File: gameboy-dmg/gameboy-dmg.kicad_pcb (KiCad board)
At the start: 2 copper layers, 82 x 63.5 mm, 29 parts, among them J1 Conn_01x02, J2 Conn_01x06, J3 Conn_01x02, U1 MCP23017_SO

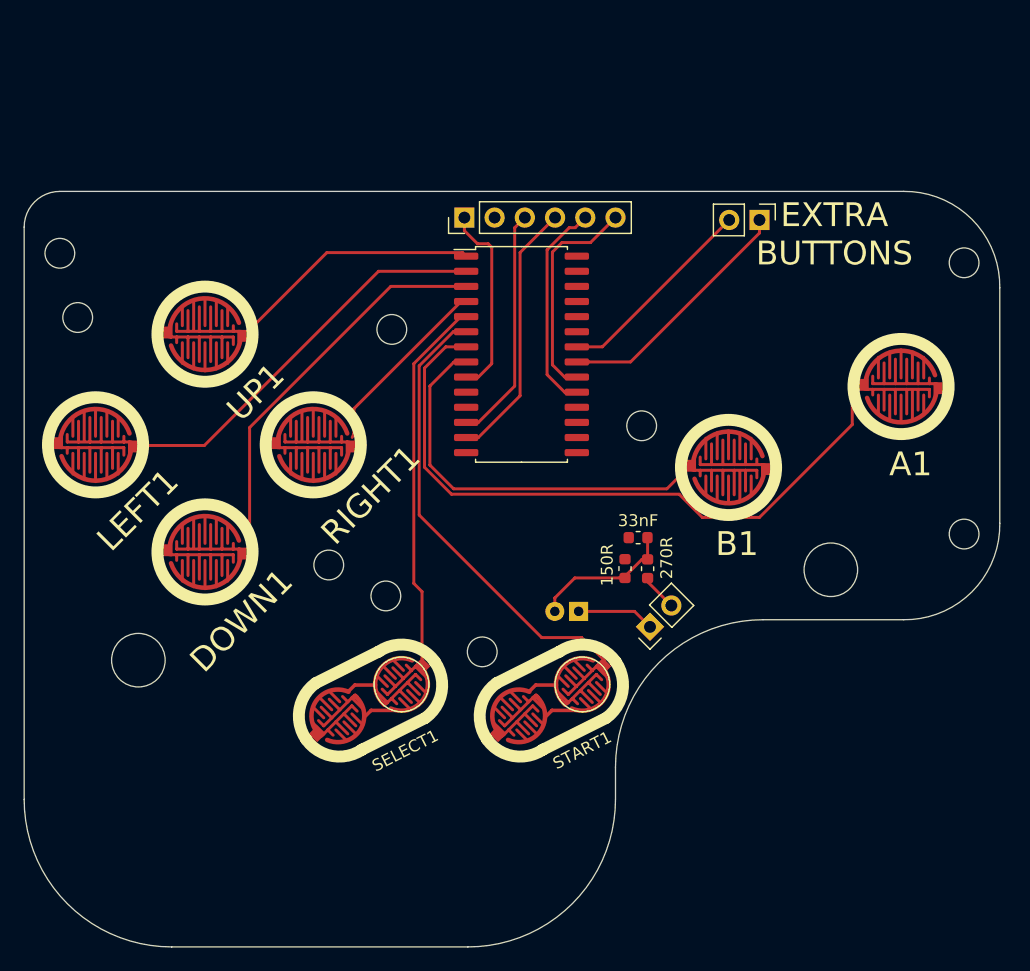
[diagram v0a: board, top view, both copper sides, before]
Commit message: Added some more bits
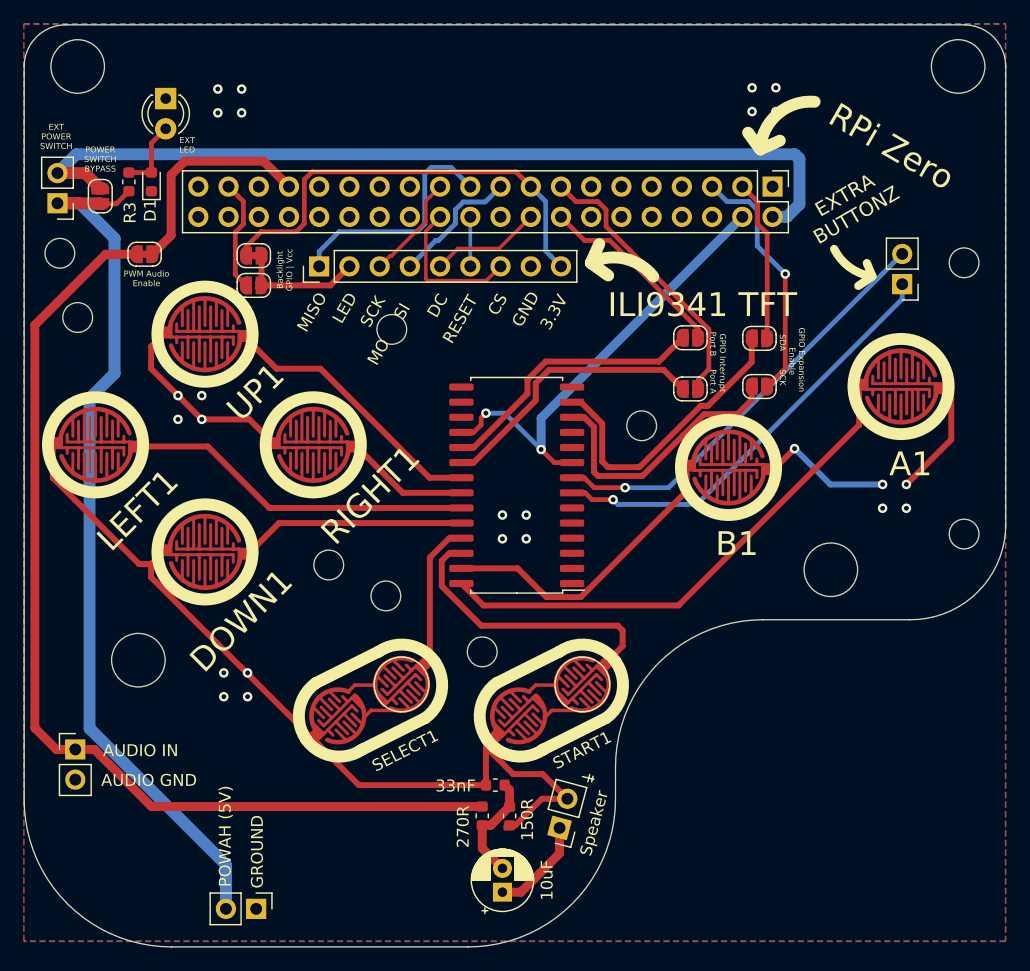
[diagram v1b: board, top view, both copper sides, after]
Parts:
- added D1: LED, LED_SMD:LED_0603_1608Metric, F.Cu at (133.7, 72.2)
- added D2: LED, LED_THT:LED_D3.0mm, F.Cu at (134.9, 65.2)
- added J4: Conn_01x02, Connector_PinHeader_2.54mm:PinHeader_1x02_P2.54mm_Vertical, F.Cu at (127.3, 119.9)
- added J5: Raspberry_Pi_2_3, Connector_PinHeader_2.54mm:PinHeader_2x20_P2.54mm_Vertical, F.Cu at (185.9, 72.6)
- added J6: Conn_01x09, Connector_PinHeader_2.54mm:PinHeader_1x09_P2.54mm_Vertical, F.Cu at (147.8, 79.3)
- added JP1: SolderJumper_2_Bridged, Jumper:SolderJumper-2_P1.3mm_Bridged_RoundedPad1.0x1.5mm, F.Cu at (133.1, 78.3)
- added JP2: SolderJumper_2_Open, Jumper:SolderJumper-2_P1.3mm_Open_RoundedPad1.0x1.5mm, F.Cu at (184.8, 89.4)
- added JP3: SolderJumper_2_Open, Jumper:SolderJumper-2_P1.3mm_Open_RoundedPad1.0x1.5mm, F.Cu at (184.8, 85.3)
- added JP4: SolderJumper_2_Open, Jumper:SolderJumper-2_P1.3mm_Open_RoundedPad1.0x1.5mm, F.Cu at (179.0, 85.3)
- added JP5: SolderJumper_2_Open, Jumper:SolderJumper-2_P1.3mm_Open_RoundedPad1.0x1.5mm, F.Cu at (179.0, 89.6)
- added JP6: SolderJumper_2_Open, Jumper:SolderJumper-2_P1.3mm_Open_RoundedPad1.0x1.5mm, F.Cu at (142.3, 80.9)
- added JP7: SolderJumper_2_Bridged, Jumper:SolderJumper-2_P1.3mm_Bridged_RoundedPad1.0x1.5mm, F.Cu at (142.3, 78.4)
- added JP8: SolderJumper_2_Open, Jumper:SolderJumper-2_P1.3mm_Open_RoundedPad1.0x1.5mm, F.Cu at (129.4, 73.4)
- added R3: R_Small, Resistor_SMD:R_0603_1608Metric, F.Cu at (131.8, 72.2)
- added REF**: MountingHole_4.5mm, MountingHole:MountingHole_4.5mm, F.Cu at (127.5, 62.5)
- added REF**: MountingHole_4.5mm, MountingHole:MountingHole_4.5mm, F.Cu at (201.5, 62.5)
- added SW1: SW_DIP_x01, Connector_PinHeader_2.54mm:PinHeader_1x02_P2.54mm_Vertical, F.Cu at (125.8, 74.0)
- C2: moved to F.Cu
- J2: value Conn_01x06 -> Conn_01x02; footprint Connector_PinHeader_2.54mm:PinHeader_1x06_P2.54mm_Vertical -> Connector_PinHeader_2.54mm:PinHeader_1x02_P2.54mm_Vertical
- moved J2 60.7 mm to (142.5, 133.3), turned to 270 degrees
- moved R1 25.0 mm to (161.5, 125.5), turned to 90 degrees
- moved C2 24.5 mm to (163.2, 131.9), turned to 90 degrees
- moved C1 24.0 mm to (162.6, 122.9)
- moved R2 23.0 mm to (163.8, 125.5), turned to 90 degrees
- moved J1 18.5 mm to (168.0, 126.5), turned to 165 degrees
- moved J3 13.2 mm to (196.8, 80.8), turned to 180 degrees
- moved U1 11.0 mm to (164.4, 97.7), turned to 180 degrees
- moved G*** 6.02 mm to (176.5, 107.0)
- moved G*** 0.22 mm to (135.9, 106.7)
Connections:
- J1 pad 2: /PWM_IN -> GND
- J2 pad 1: +5V -> GND
- J2 pad 2: GND -> Net-(J2-Pad2)
- U1 pad 1: /UP -> Net-(U1-Pad1)
- U1 pad 12: Net-(J2-Pad3) -> /GPIO_SCK
- U1 pad 13: Net-(J2-Pad4) -> /GPIO_SDA
- U1 pad 19: Net-(J2-Pad5) -> /GPIO_INTB
- U1 pad 2: /LEFT -> Net-(U1-Pad2)
- U1 pad 20: Net-(J2-Pad6) -> /GPIO_INTA
- U1 pad 21: Net-(J3-Pad1) -> /UP
- U1 pad 22: Net-(J3-Pad2) -> /RIGHT
- U1 pad 23: Net-(U1-Pad23) -> /LEFT
- U1 pad 24: Net-(U1-Pad24) -> /DOWN
- U1 pad 25: Net-(U1-Pad25) -> /SELECT
- U1 pad 26: Net-(U1-Pad26) -> /START
- U1 pad 27: Net-(U1-Pad27) -> /B
- U1 pad 28: Net-(U1-Pad28) -> /A
- U1 pad 3: /DOWN -> Net-(U1-Pad3)
- U1 pad 4: /RIGHT -> Net-(U1-Pad4)
- U1 pad 5: /SELECT -> Net-(U1-Pad5)
- U1 pad 6: /START -> Net-(U1-Pad6)
- U1 pad 7: /A -> Net-(J3-Pad1)
- U1 pad 8: /B -> Net-(J3-Pad2)
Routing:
- net GND: track 0.00 -> 108.1 mm, vias 0 -> 25
- net +5V: track 16.4 -> 112.4 mm, vias 0 -> 2
- net /PWM_IN: track 3.13 -> 85.2 mm
- net Net-(J2-Pad2): track 0.00 -> 74.4 mm
- net +3V3: track 0.00 -> 37.7 mm
- net /GPIO_SDA: track 0.00 -> 24.9 mm
- net /GPIO_INTA_PI: track 0.00 -> 23.6 mm
- net /GPIO_INTA: track 0.00 -> 23.3 mm
- net /GPIO_SCK: track 0.00 -> 23.1 mm
- net /GPIO_INTB: track 0.00 -> 23.1 mm
- net Net-(J2-Pad4): track 22.2 -> 0.00 mm
- net /GPIO_SCK_PI: track 0.00 -> 21.1 mm, vias 0 -> 1
- net /TFT_MISO: track 0.00 -> 20.0 mm
- net Net-(J2-Pad3): track 19.9 -> 0.00 mm
- net /SELECT: track 31.2 -> 12.2 mm
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- added copper zone on B.Cu, net GND
- added copper zone on F.Cu, net GND
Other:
- board size 82 x 63.5 mm -> 82.5 x 77.5 mm
- net class Default: trace_width 0.25 -> 0.3
- board text added: "3.3V"
- board text added: "AUDIO GND"
- board text added: "AUDIO IN"
- board text added: "Backlight GPIO | Vcc"
- board text added: "CS"
- board text added: "DC"
- board text added: "EXT LED"
- board text added: "EXT POWER SWITCH"
- board text added: "EXTRA BUTTONZ"
- board text added: "GND"
- board text added: "GPIO Expansion Enable SDA SCK"
- board text added: "GPIO Interrupt Port B Port A"
- board text added: "ILI9341 TFT"
- board text added: "LED"
- board text added: "MISO"
- board text added: "MO SI"
- board text added: "POWAH (5V)"
- board text added: "POWER SWITCH BYPASS"
- board text added: "PWM Audio Enable"
- board text added: "RESET"
- board text added: "RPi Zero"
- board text added: "Raspberry Pi Zero Gameboy DMG Shield by Alex Hoffman"
- board text added: "Speaker"
- board text added: "TUX"
- board text removed: "5V POWAH"
- board text removed: "EXTRA BUTTONS"
- board text removed: "INTERRUPT A"
- board text removed: "INTERRUPT B"
- board text removed: "SDA"
